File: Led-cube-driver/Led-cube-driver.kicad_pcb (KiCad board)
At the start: 2 copper layers, 31 parts, among them J1 Diodes-input, J2 Vin, J3 Diodes-output, J4 Layers-input, J5 Layers-output, Q1 BC547, Q2 BC547, Q3 BC547, Q4 BC547, U1 74HC164, U2 74HC164

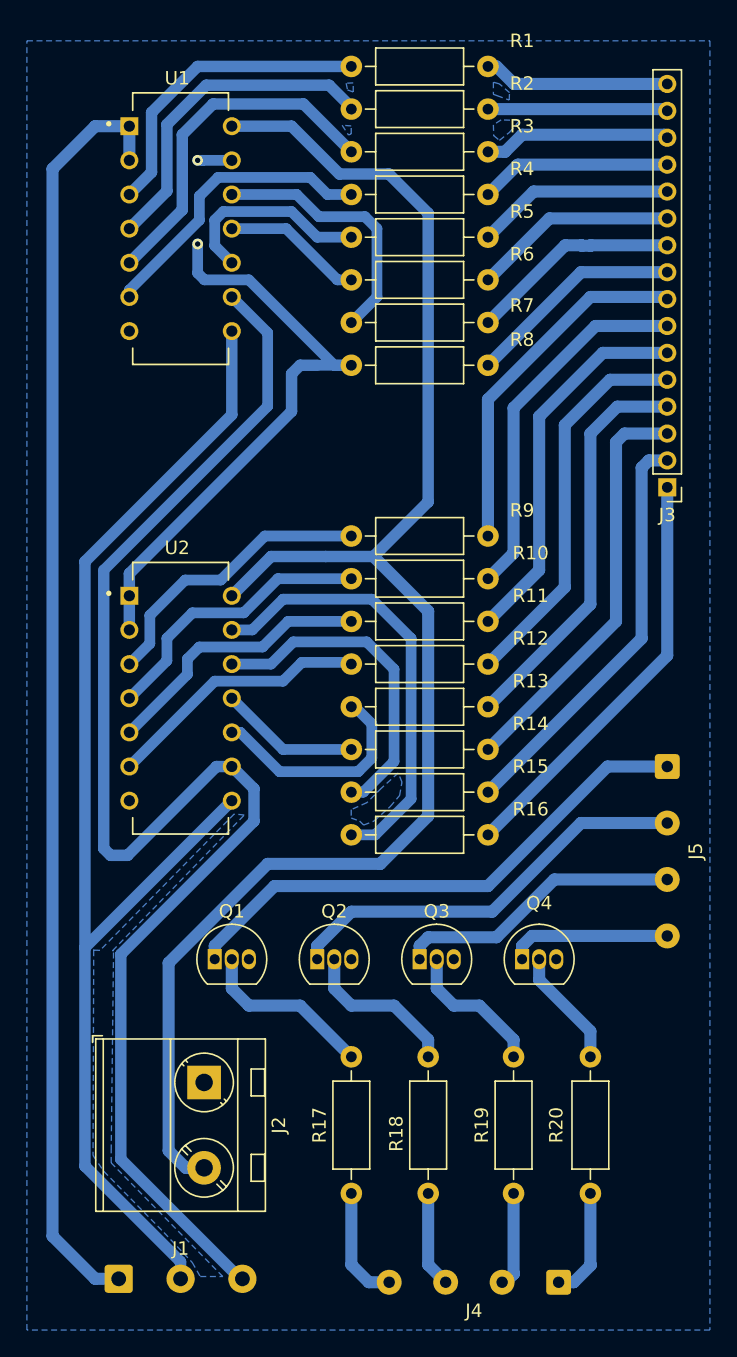
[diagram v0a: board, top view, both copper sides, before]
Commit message: done
done
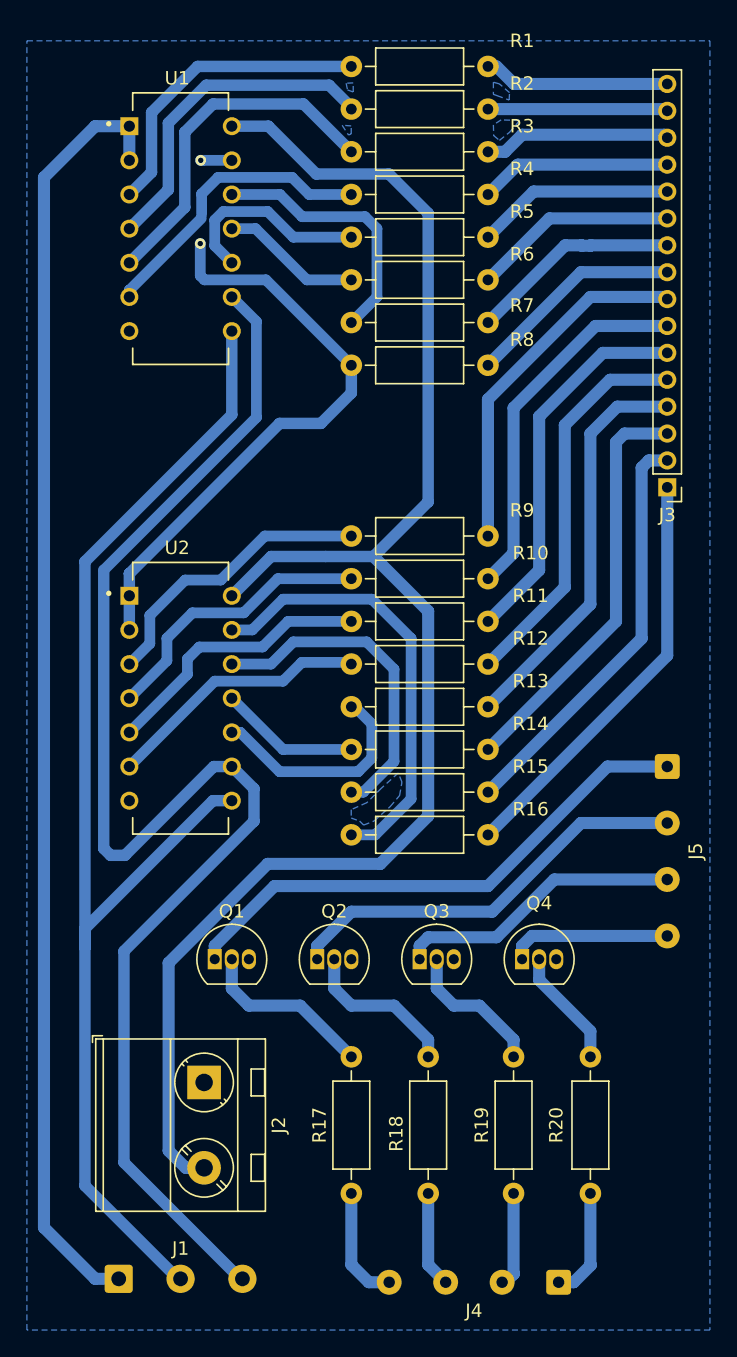
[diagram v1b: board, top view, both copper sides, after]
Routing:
- net Net-(J1-Pad2): track 93.4 -> 94.3 mm
- net Net-(J1-Pad3): track 106.4 -> 105.5 mm
- net Net-(R8-Pad1): track 47.7 -> 47.0 mm
- net Net-(J1-Pad1): track 95.2 -> 95.7 mm
